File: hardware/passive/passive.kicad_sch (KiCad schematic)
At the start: 7 parts, among them J1 i/O, J2 Conn 1, J3 Conn 2

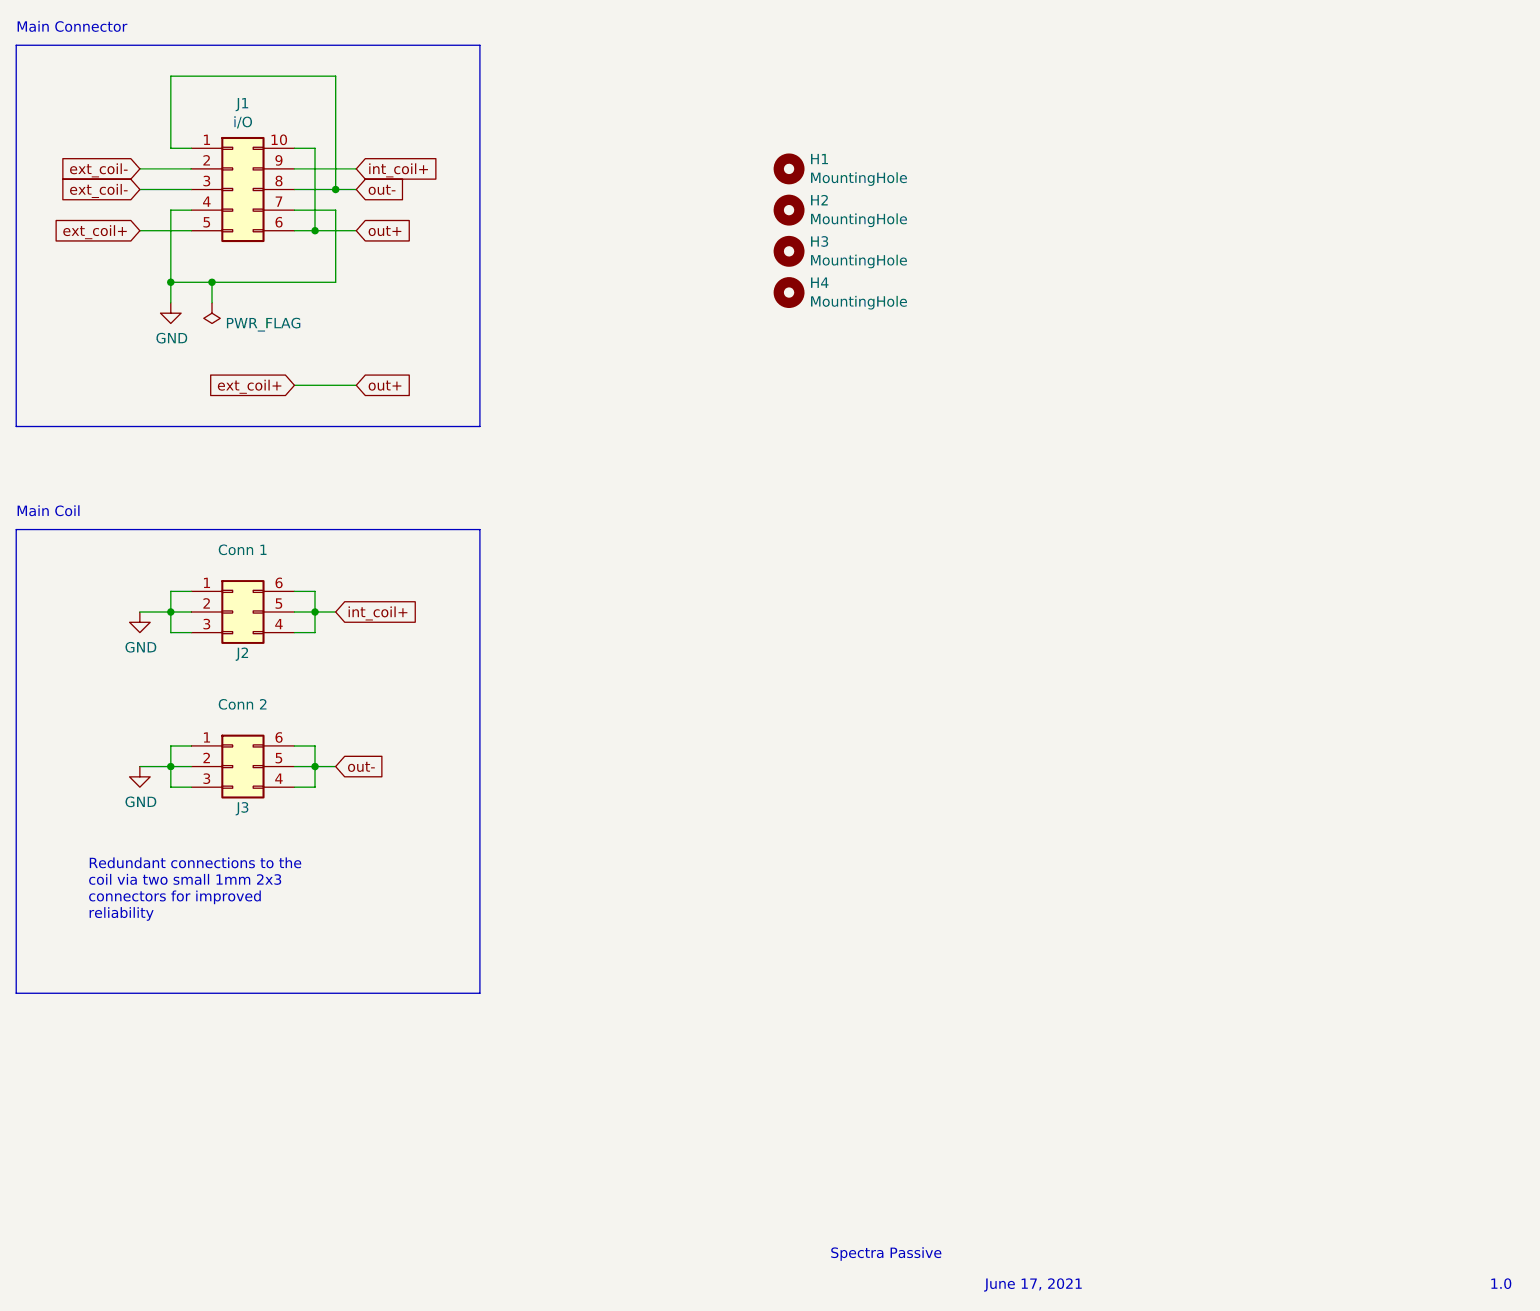
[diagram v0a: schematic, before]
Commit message: v2.0 layout
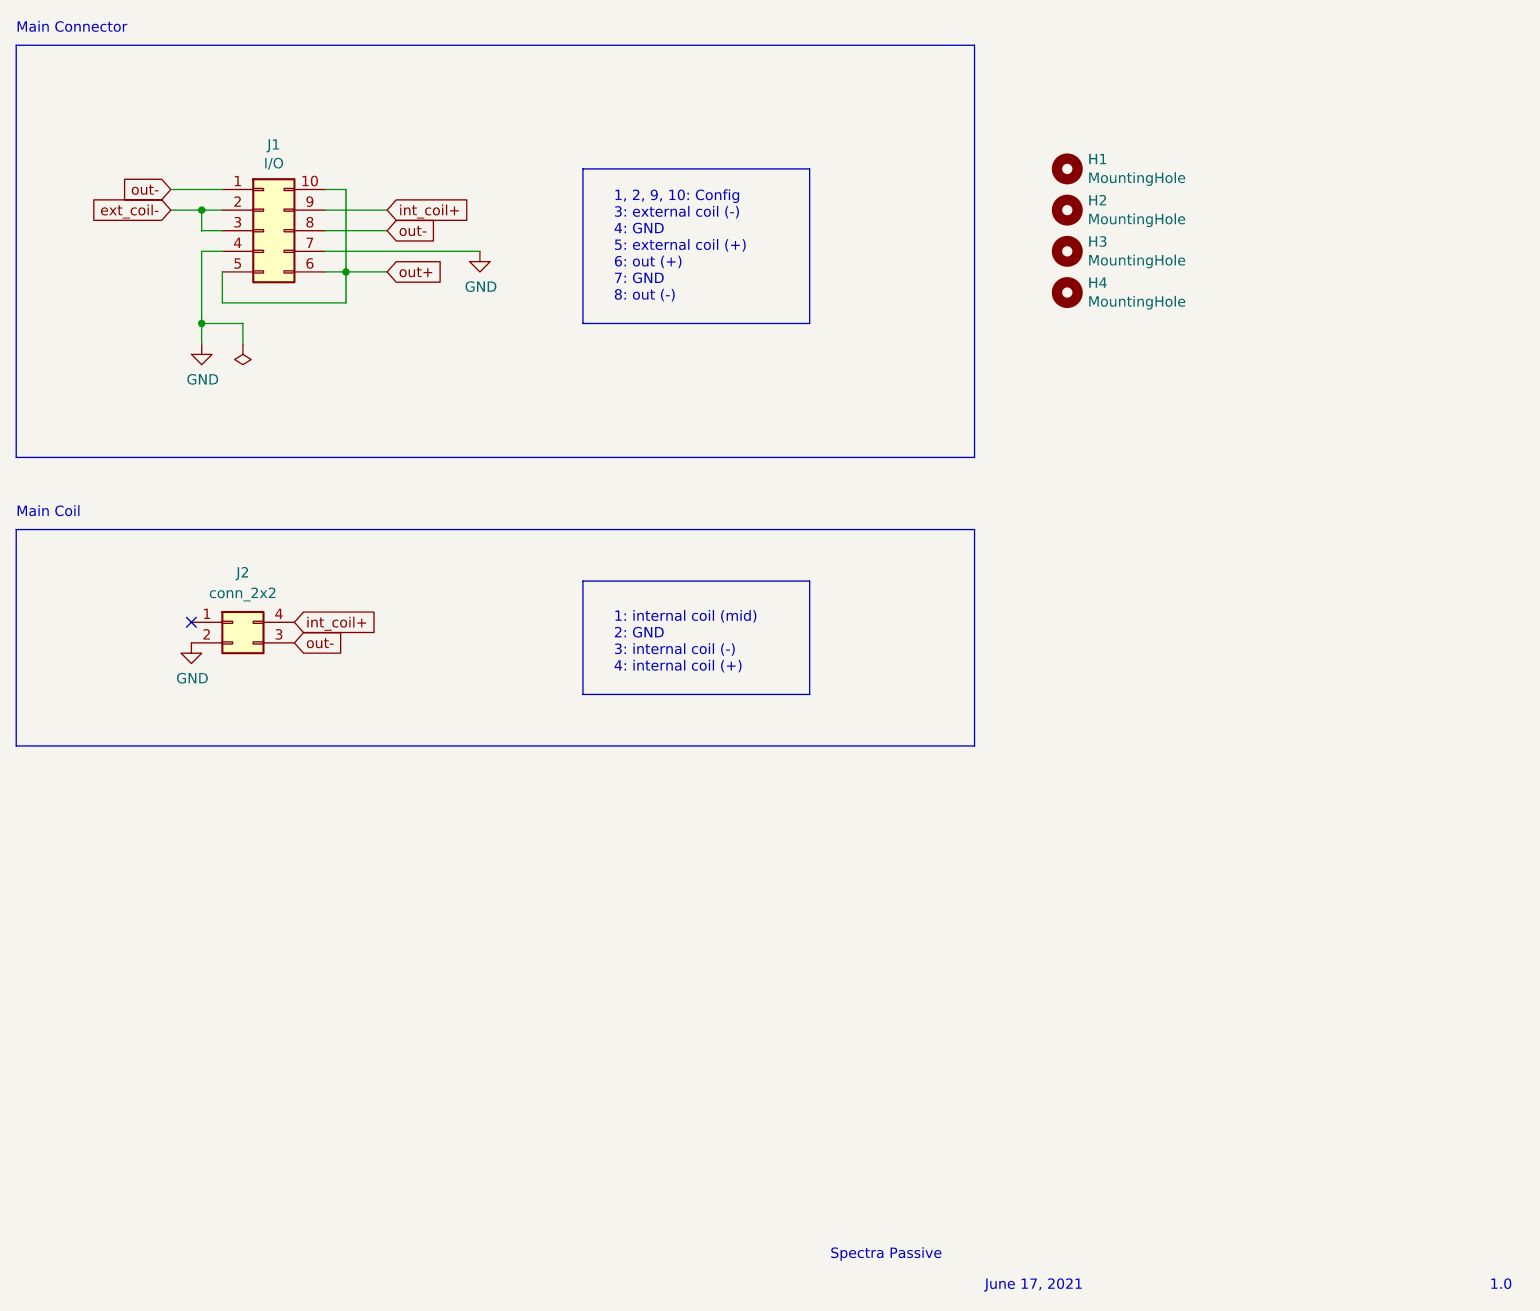
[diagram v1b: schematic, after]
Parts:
- removed J2: Conn 1, cycfi_library:pin_socket_2x3p_1.00mm_smd_vertical, symbol Connector_Generic:Conn_02x03_Counter_Clockwise
- removed J3: Conn 2, cycfi_library:pin_socket_2x3p_1.00mm_smd_vertical, symbol Connector_Generic:Conn_02x03_Counter_Clockwise
- added J2: conn_2x2, cycfi_library:pin_socket_2x2p_2.00mm_smd_vertical, symbol Connector_Generic:Conn_02x02_Counter_Clockwise
- J1: value i/O -> I/O
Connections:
- net GND: now also J2.2 (Pin_2)
- net int_coil+: now also J2.4 (Pin_4)
- net out-: now also J2.3 (Pin_3)
- net ext_coil+ renamed out+
- no-connect marks 0 -> 1
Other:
- note added: "1, 2, 9, 10: Config 3: external coil (-) 4: GND 5: external coil (+) 6: out (+) 7: GND 8: out (-)"
- note added: "1: internal coil (mid) 2: GND 3: internal coil (-) 4: internal coil (+)"
- note removed: "Redundant connections to the coil via two small 1mm 2x3 connectors for improved reliability"
- moved on the sheet: H1, H2, H3, H4, J1
